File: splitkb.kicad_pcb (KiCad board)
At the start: 2 copper layers, 166.4 x 132.1 mm, 151 parts, among them J1 MJ-4PP-9, K1 KEYSW, SW1 SW_PUSH, SW10 SW_PUSH, SW11 SW_PUSH, SW12 SW_PUSH, SW13 SW_PUSH, SW14 SW_PUSH, SW15 SW_PUSH, SW16 SW_PUSH, SW17 SW_PUSH, SW18 SW_PUSH, SW19 SW_PUSH, SW2 SW_PUSH, SW20 SW_PUSH, SW21 SW_PUSH, SW22 SW_PUSH, SW23 SW_PUSH, SW24 SW_PUSH, SW25 SW_PUSH, SW26 SW_PUSH, SW27 SW_PUSH, SW28 SW_PUSH, SW29 SW_PUSH, SW3 SW_PUSH, SW30 SW_PUSH, SW31 SW_PUSH, SW32 SW_PUSH, SW33 SW_PUSH, SW34 SW_PUSH, SW35 SW_PUSH, SW4 SW_PUSH, SW5 SW_PUSH, SW6 SW_PUSH, SW7 SW_PUSH, SW8 SW_PUSH, SW9 SW_PUSH, U1 ProMicro

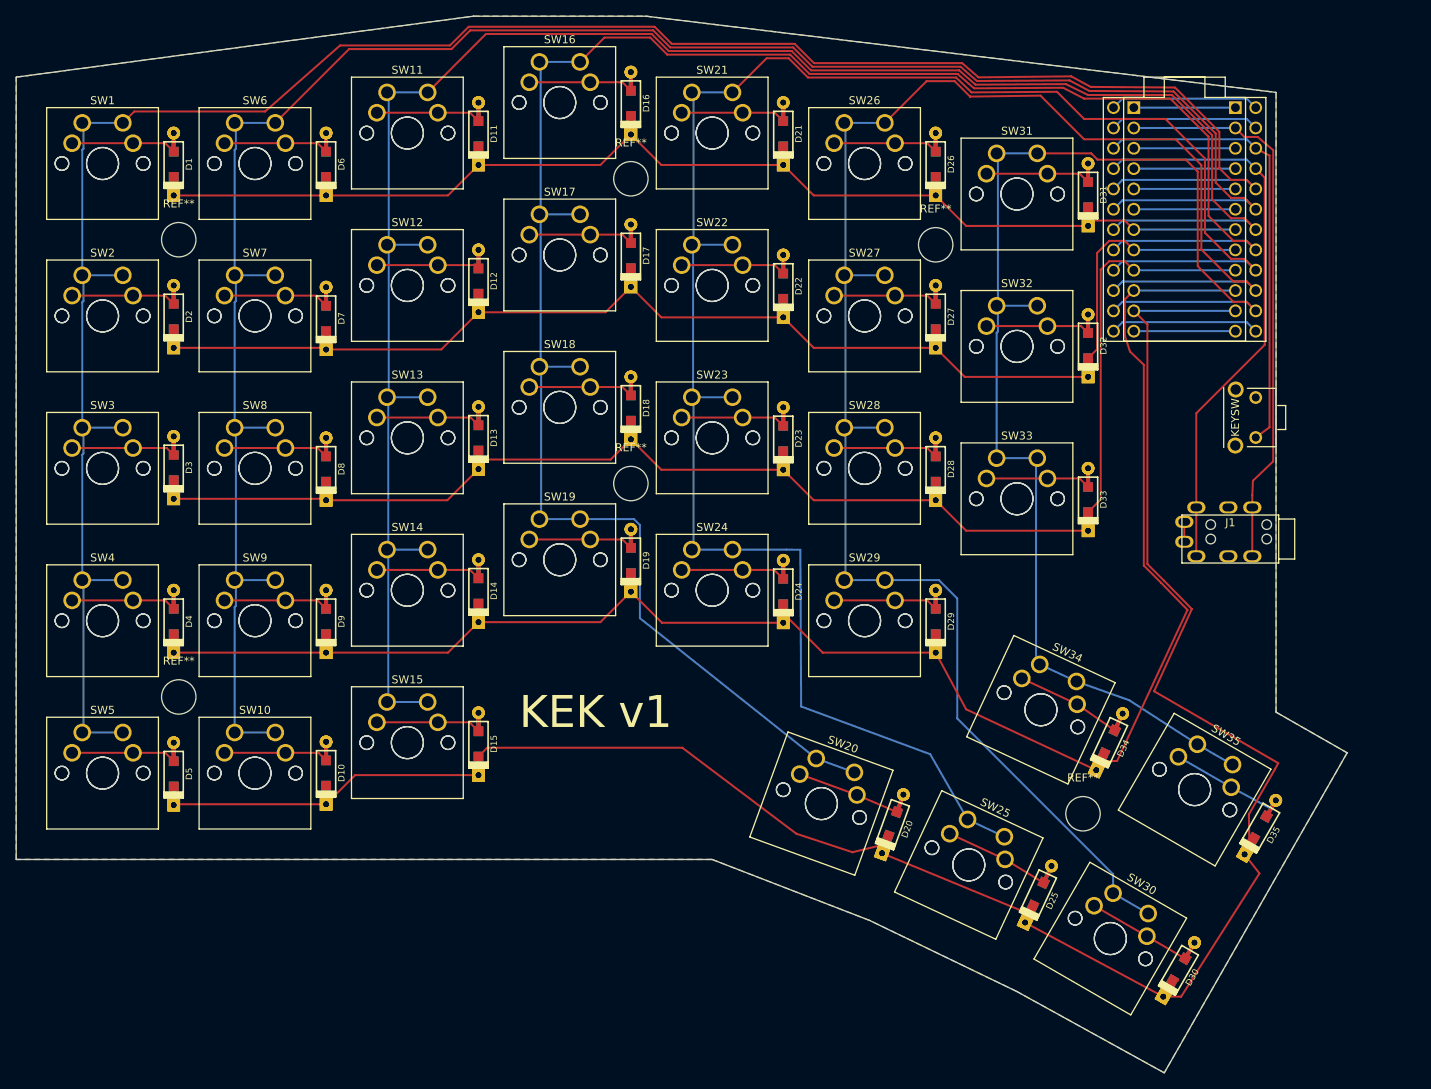
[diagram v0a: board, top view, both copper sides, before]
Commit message: new rev
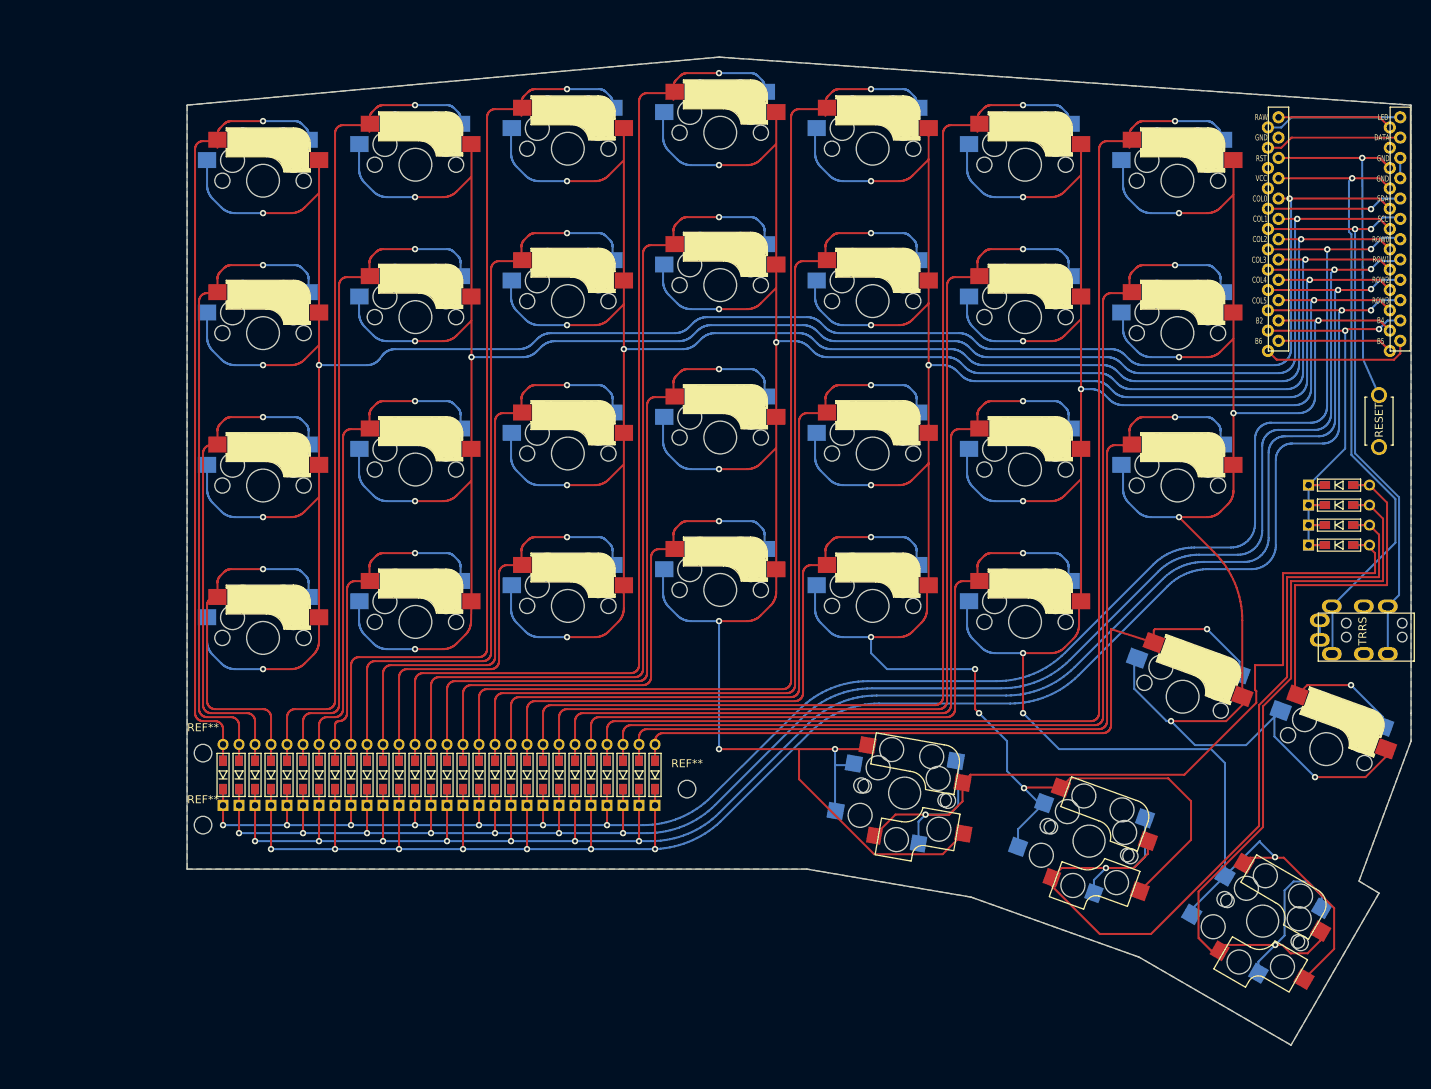
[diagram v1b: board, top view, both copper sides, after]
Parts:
- removed the D1 at (36.8, 50.9) (x2)
- removed the D10 at (55.9, 127.0) (x2)
- removed the D11 at (74.9, 47.1) (x2)
- removed the D12 at (74.9, 65.5) (x2)
- removed the D13 at (74.9, 85.1) (x2)
- removed the D14 at (74.9, 104.2) (x2)
- removed the D15 at (74.9, 123.3) (x2)
- removed the D16 at (94.0, 43.3) (x2)
- removed the D17 at (94.0, 62.3) (x2)
- removed the D18 at (94.0, 81.4) (x2)
- removed the D19 at (94.0, 100.4) (x2)
- removed the D2 at (36.8, 69.9) (x2)
- removed the D20 at (126.7, 133.3) (x2)
- removed the D21 at (113.0, 47.1) (x2)
- removed the D22 at (113.0, 66.1) (x2)
- removed the D23 at (113.0, 85.2) (x2)
- removed the D24 at (113.0, 104.3) (x2)
- removed the D25 at (144.9, 142.1) (x2)
- removed the D26 at (132.1, 50.9) (x2)
- removed the D27 at (132.1, 69.9) (x2)
- removed the D28 at (132.1, 89.0) (x2)
- removed the D29 at (132.1, 108.0) (x2)
- removed the D3 at (36.8, 88.8) (x2)
- removed the D30 at (162.5, 151.6) (x2)
- removed the D31 at (151.1, 54.7) (x2)
- removed the D32 at (151.1, 73.6) (x2)
- removed D33 (x2), D34 (x2), D35 (x2): D, keyboard_parts:D_SOD123_axial
- removed the D4 at (36.8, 108.0) (x2)
- removed the D5 at (36.8, 127.1) (x2)
- removed the D6 at (55.9, 50.9) (x2)
- removed the D7 at (55.9, 70.2) (x2)
- removed the D8 at (55.9, 89.0) (x2)
- removed the D9 at (55.9, 108.0) (x2)
- removed the J1 at (168.9, 95.9)
- removed the J1 at (168.9, 97.8)
- removed the REF** at (37.5, 117.5)
- removed the REF** at (37.5, 60.3)
- removed the REF** at (94.0, 90.8)
- removed the REF** at (94.0, 52.7)
- removed the REF** at (132.1, 61.0)
- removed the REF** at (150.5, 132.1)
- removed the SW1 at (25.4, 45.7)
- removed the SW1 at (30.5, 45.7)
- removed the SW10 at (44.5, 121.9)
- removed the SW10 at (49.5, 121.9)
- removed the SW11 at (63.5, 41.9)
- removed the SW11 at (68.6, 41.9)
- removed the SW12 at (63.5, 61.0)
- removed the SW12 at (68.6, 61.0)
- removed the SW13 at (63.5, 80.0)
- removed the SW13 at (68.6, 80.0)
- removed the SW14 at (63.5, 99.1)
- removed the SW14 at (68.6, 99.1)
- removed the SW15 at (63.5, 118.1)
- removed the SW15 at (68.6, 118.1)
- removed the SW16 at (82.5, 38.1)
- removed the SW16 at (87.6, 38.1)
- removed the SW17 at (82.5, 57.1)
- removed the SW17 at (87.6, 57.1)
- removed the SW18 at (82.5, 76.2)
- removed the SW18 at (87.6, 76.2)
- removed the SW19 at (82.5, 95.2)
- removed the SW19 at (87.6, 95.2)
- removed the SW2 at (25.4, 64.8)
- removed the SW2 at (30.5, 64.8)
- removed the SW20 at (117.1, 125.2)
- removed the SW20 at (121.9, 126.9)
- removed the SW21 at (101.6, 41.9)
- removed the SW21 at (106.7, 41.9)
- removed the SW22 at (101.6, 61.0)
- removed the SW22 at (106.7, 61.0)
- removed the SW23 at (106.7, 80.0)
- removed the SW23 at (101.6, 80.0)
- removed the SW24 at (101.6, 99.1)
- removed the SW24 at (106.7, 99.1)
- removed the SW25 at (136.1, 132.8)
- removed the SW25 at (140.7, 135.0)
- removed the SW26 at (120.7, 45.7)
- removed the SW26 at (125.7, 45.7)
- removed the SW27 at (120.7, 64.8)
- removed the SW27 at (125.7, 64.8)
- removed the SW28 at (120.7, 83.8)
- removed the SW28 at (125.7, 83.8)
- removed the SW29 at (120.7, 102.9)
- removed the SW29 at (125.7, 102.9)
- removed the SW3 at (25.4, 83.8)
- removed the SW3 at (30.5, 83.8)
- removed the SW30 at (154.3, 142.0)
- removed the SW30 at (158.6, 144.6)
- removed the SW31 at (139.7, 49.5)
- removed the SW31 at (144.8, 49.5)
- removed the SW32 at (139.7, 68.6)
- removed the SW32 at (144.8, 68.6)
- removed SW33 (x2), SW34 (x2), SW35 (x2): SW_PUSH, Button_Switch_Keyboard:SW_Cherry_MX_1.00u_PCB
- removed the SW4 at (25.4, 102.9)
- removed the SW4 at (30.5, 102.9)
- removed the SW5 at (25.4, 121.9)
- removed the SW5 at (30.5, 121.9)
- removed the SW6 at (44.5, 45.7)
- removed the SW6 at (49.5, 45.7)
- removed the SW7 at (44.5, 64.8)
- removed the SW7 at (49.5, 64.8)
- removed the SW8 at (44.5, 83.8)
- removed the SW8 at (49.5, 83.8)
- removed the SW9 at (44.5, 102.9)
- removed the SW9 at (49.5, 102.9)
- removed the U1 at (164.5, 57.8)
- removed the U1 at (161.9, 57.8)
- added D1: D, kbd:D3_TH_SMD, F.Cu at (43.0, 127.2)
- added D10: D, kbd:D3_TH_SMD, F.Cu at (61.0, 127.2)
- added D11: D, kbd:D3_TH_SMD, F.Cu at (63.0, 127.2)
- added D12: D, kbd:D3_TH_SMD, F.Cu at (65.0, 127.2)
- added D13: D, kbd:D3_TH_SMD, F.Cu at (67.0, 127.2)
- added D14: D, kbd:D3_TH_SMD, F.Cu at (69.0, 127.2)
- added D15: D, kbd:D3_TH_SMD, F.Cu at (71.0, 127.2)
- added D16: D, kbd:D3_TH_SMD, F.Cu at (73.0, 127.2)
- added D17: D, kbd:D3_TH_SMD, F.Cu at (182.5, 98.5)
- added D18: D, kbd:D3_TH_SMD, F.Cu at (75.0, 127.2)
- added D19: D, kbd:D3_TH_SMD, F.Cu at (77.0, 127.2)
- added D2: D, kbd:D3_TH_SMD, F.Cu at (45.0, 127.2)
- added D20: D, kbd:D3_TH_SMD, F.Cu at (79.0, 127.2)
- added D21: D, kbd:D3_TH_SMD, F.Cu at (81.0, 127.2)
- added D22: D, kbd:D3_TH_SMD, F.Cu at (182.5, 96.0)
- added D23: D, kbd:D3_TH_SMD, F.Cu at (83.0, 127.2)
- added D24: D, kbd:D3_TH_SMD, F.Cu at (85.0, 127.2)
- added D25: D, kbd:D3_TH_SMD, F.Cu at (87.0, 127.2)
- added D26: D, kbd:D3_TH_SMD, F.Cu at (89.0, 127.2)
- added D27: D, kbd:D3_TH_SMD, F.Cu at (182.5, 93.5)
- added D28: D, kbd:D3_TH_SMD, F.Cu at (91.0, 127.2)
- added D29: D, kbd:D3_TH_SMD, F.Cu at (93.0, 127.2)
- added D3: D, kbd:D3_TH_SMD, F.Cu at (47.0, 127.2)
- added D30: D, kbd:D3_TH_SMD, F.Cu at (95.0, 127.2)
- added D31: D, kbd:D3_TH_SMD, F.Cu at (97.0, 127.2)
- added D32: D, kbd:D3_TH_SMD, F.Cu at (182.5, 91.0)
- added D4: D, kbd:D3_TH_SMD, F.Cu at (49.0, 127.2)
- added D5: D, kbd:D3_TH_SMD, F.Cu at (51.0, 127.2)
- added D6: D, kbd:D3_TH_SMD, F.Cu at (53.0, 127.2)
- added D7: D, kbd:D3_TH_SMD, F.Cu at (55.0, 127.2)
- added D8: D, kbd:D3_TH_SMD, F.Cu at (57.0, 127.2)
- added D9: D, kbd:D3_TH_SMD, F.Cu at (59.0, 127.2)
- added J1: MJ-4PP-9, kbd:MJ-4PP-9, F.Cu at (191.9, 110.0)
- added REF**: MountingHole_2.2mm_M2, MountingHole:MountingHole_2.2mm_M2, F.Cu at (101.0, 129.0)
- added REF**: MountingHole_2.2mm_M2, MountingHole:MountingHole_2.2mm_M2, F.Cu at (40.5, 133.5)
- added REF**: MountingHole_2.2mm_M2, MountingHole:MountingHole_2.2mm_M2, F.Cu at (40.5, 124.5)
- added SW1: SW_PUSH, kbd:CherryMX_Hotswap, F.Cu at (48.0, 53.0)
- added SW10: SW_PUSH, kbd:CherryMX_Hotswap, F.Cu at (86.1, 68.0)
- added SW11: SW_PUSH, kbd:CherryMX_Hotswap, F.Cu at (86.1, 87.0)
- added SW12: SW_PUSH, kbd:CherryMX_Hotswap, F.Cu at (86.1, 106.1)
- added SW13: SW_PUSH, kbd:CherryMX_Hotswap, F.Cu at (105.2, 47.0)
- added SW14: SW_PUSH, kbd:CherryMX_Hotswap, F.Cu at (105.2, 66.0)
- added SW15: SW_PUSH, kbd:CherryMX_Hotswap, F.Cu at (105.2, 85.0)
- added SW16: SW_PUSH, kbd:CherryMX_Hotswap, F.Cu at (105.2, 104.1)
- added SW17: SW_PUSH, kbd:CherryMX_Choc_Hotswap, F.Cu at (128.2, 129.5)
- added SW18: SW_PUSH, kbd:CherryMX_Hotswap, F.Cu at (124.2, 49.0)
- added SW19: SW_PUSH, kbd:CherryMX_Hotswap, F.Cu at (124.2, 68.0)
- added SW2: SW_PUSH, kbd:CherryMX_Hotswap, F.Cu at (48.0, 72.0)
- added SW20: SW_PUSH, kbd:CherryMX_Hotswap, F.Cu at (124.2, 87.0)
- added SW21: SW_PUSH, kbd:CherryMX_Hotswap, F.Cu at (124.2, 106.1)
- added SW22: SW_PUSH, kbd:CherryMX_Choc_Hotswap, F.Cu at (151.3, 135.5)
- added SW23: SW_PUSH, kbd:CherryMX_Hotswap, F.Cu at (143.2, 51.0)
- added SW24: SW_PUSH, kbd:CherryMX_Hotswap, F.Cu at (143.2, 70.0)
- added SW25: SW_PUSH, kbd:CherryMX_Hotswap, F.Cu at (143.2, 89.0)
- added SW26: SW_PUSH, kbd:CherryMX_Hotswap, F.Cu at (143.2, 108.1)
- added SW27: SW_PUSH, kbd:CherryMX_Choc_Hotswap, F.Cu at (172.9, 145.5)
- added SW28: SW_PUSH, kbd:CherryMX_Hotswap, F.Cu at (162.3, 53.0)
- added SW29: SW_PUSH, kbd:CherryMX_Hotswap, F.Cu at (162.3, 72.0)
- added SW3: SW_PUSH, kbd:CherryMX_Hotswap, F.Cu at (48.0, 91.0)
- added SW30: SW_PUSH, kbd:CherryMX_Hotswap, F.Cu at (162.3, 91.0)
- added SW31: SW_PUSH, kbd:CherryMX_Hotswap, F.Cu at (162.9, 117.5)
- added SW32: SW_PUSH, kbd:CherryMX_Hotswap, F.Cu at (180.9, 124.0)
- added SW4: SW_PUSH, kbd:CherryMX_Hotswap, F.Cu at (48.0, 110.1)
- added SW5: SW_PUSH, kbd:CherryMX_Hotswap, F.Cu at (67.0, 51.0)
- added SW6: SW_PUSH, kbd:CherryMX_Hotswap, F.Cu at (67.0, 70.0)
- added SW7: SW_PUSH, kbd:CherryMX_Hotswap, F.Cu at (67.0, 89.0)
- added SW8: SW_PUSH, kbd:CherryMX_Hotswap, F.Cu at (67.0, 108.1)
- added SW9: SW_PUSH, kbd:CherryMX_Hotswap, F.Cu at (86.1, 49.0)
- added U1: ProMicro, kbd:ProMicro_v2, F.Cu at (182.5, 59.5)
- K1: footprint keyboard_parts:SW_TACT_TH_HORIZ_LOW -> kbd:ResetSW; moved to B.Cu
- moved K1 15.4 mm to (187.5, 83.0)
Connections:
- K1 pad 1: GND -> reset
- K1 pad 2: reset -> GND
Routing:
- net row4: track 252.3 -> 62.1 mm, vias 0 -> 2
- net Net-(D28-Pad2): track 13.1 -> 160.3 mm, vias 0 -> 1
- net Net-(D23-Pad2): track 13.1 -> 151.3 mm, vias 0 -> 1
- net Net-(D18-Pad2): track 13.1 -> 142.2 mm, vias 0 -> 1
- net Net-(D29-Pad2): track 13.1 -> 139.3 mm, vias 0 -> 1
- net Net-(D13-Pad2): track 13.1 -> 133.2 mm, vias 0 -> 1
- net Net-(D24-Pad2): track 13.2 -> 130.2 mm, vias 0 -> 1
- net Net-(D19-Pad2): track 13.1 -> 121.2 mm, vias 0 -> 1
- net Net-(D9-Pad2): track 13.1 -> 120.1 mm, vias 0 -> 1
- net row0: track 141.3 -> 247.7 mm, vias 0 -> 9
- net Net-(D22-Pad2): track 13.1 -> 119.0 mm, vias 0 -> 1
- net Net-(D30-Pad2): track 13.2 -> 118.3 mm, vias 0 -> 1
- net Net-(D27-Pad2): track 13.1 -> 112.8 mm, vias 0 -> 1
- net Net-(D14-Pad2): track 13.1 -> 112.1 mm, vias 0 -> 1
- net row1: track 154.3 -> 251.7 mm, vias 0 -> 9
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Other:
- board size 166.4 x 132.1 mm -> 153 x 123.5 mm
- net class Default: trace_width 0.25 -> 0.254
- net class Power added: clearance 0.2, trace_width 0.381, via_dia 0.8, via_drill 0.4
- board text removed: "KEK v1"
